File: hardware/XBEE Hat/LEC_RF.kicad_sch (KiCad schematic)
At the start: 6 parts, among them J1 Conn_Coaxial_Small, J2 Conn_01x04, U1 XBee_SMT, U2 TLV1117-33

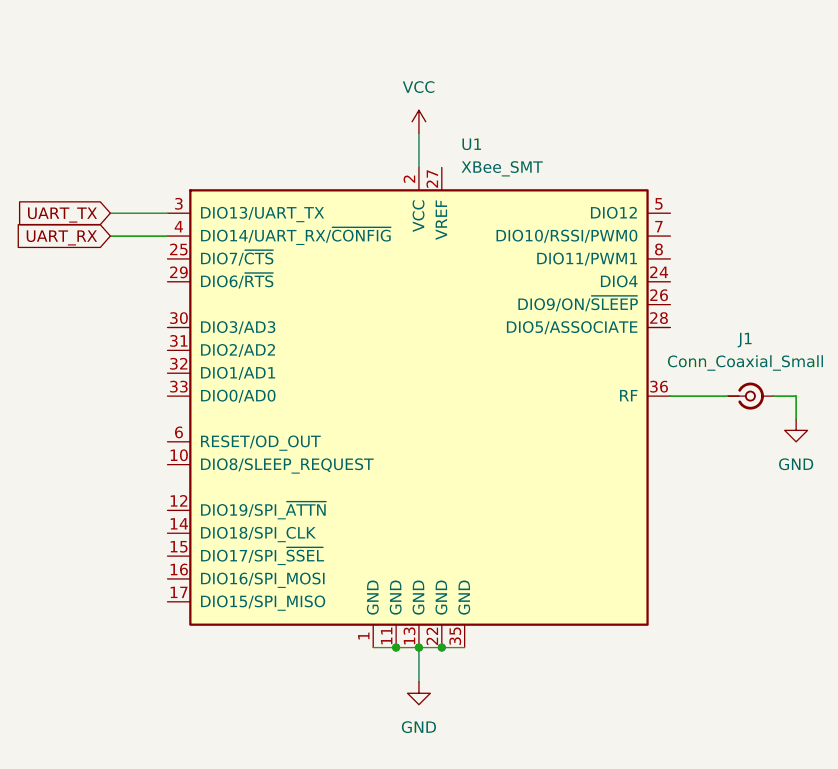
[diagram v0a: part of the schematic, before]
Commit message: Push of most recent schematic and PCB
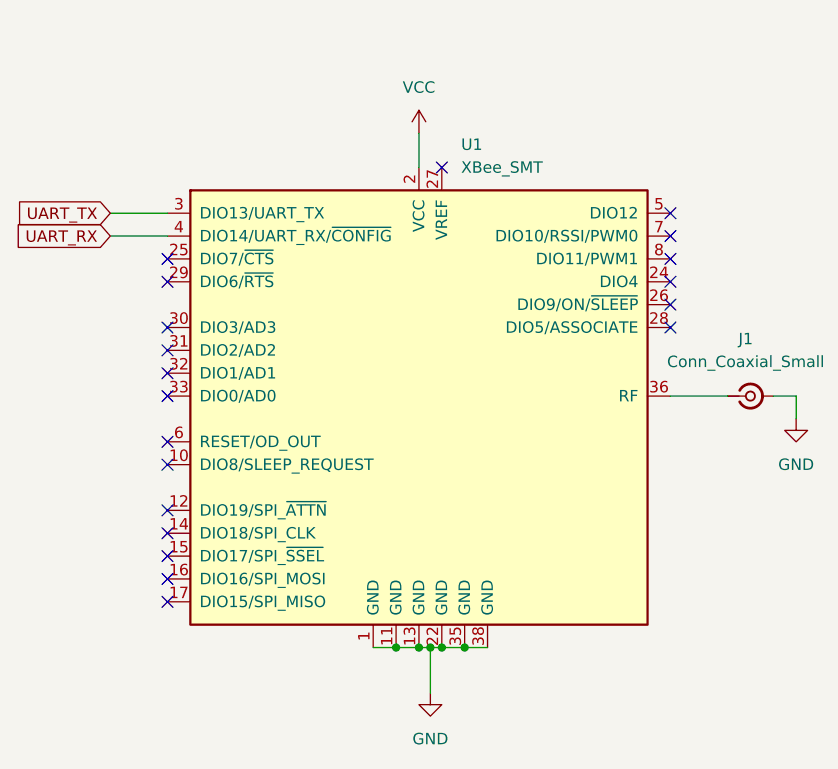
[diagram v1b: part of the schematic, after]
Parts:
- C1, C2: footprint Capacitor_SMD:C_0805_2012Metric -> Capacitor_SMD:C_0603_1608Metric
- U1: footprint RF_Module:Digi_XBee_SMT -> Custom:XBEE_GND_PAD
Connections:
- net GND: now also U1.38 (GND)
- no-connect marks 0 -> 20
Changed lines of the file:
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@@
 	(paper "A4")
+	(junction
+		(at 223.52 109.22)
+		(diameter 0)
+		(color 0 0 0 0)
+	)
+	(junction
+		(at 219.71 109.22)
+		(diameter 0)
+		(color 0 0 0 0)
+	)
 	(junction
 		(at 220.98 109.22)
@@
 		(color 0 0 0 0)
 	)
+	(no_connect
+		(at 190.5 99.06)
+	)
+	(no_connect
+		(at 190.5 93.98)
+	)
+	(no_connect
+		(at 190.5 88.9)
+	)
+	(no_connect
+		(at 190.5 96.52)
+	)
+	(no_connect
+		(at 220.98 55.88)
+	)
+	(no_connect
+		(at 190.5 68.58)
+	)
+	(no_connect
+		(at 246.38 60.96)
+	)
+	(no_connect
+		(at 246.38 63.5)
+	)
+	(no_connect
+		(at 246.38 71.12)
+	)
+	(no_connect
+		(at 190.5 101.6)
+	)
+	(no_connect
+		(at 246.38 68.58)
+	)
+	(no_connect
+		(at 190.5 66.04)
+	)
+	(no_connect
+		(at 190.5 81.28)
+	)
+	(no_connect
+		(at 190.5 73.66)
+	)
+	(no_connect
+		(at 246.38 73.66)
+	)
+	(no_connect
+		(at 246.38 66.04)
+	)
+	(no_connect
+		(at 190.5 76.2)
+	)
+	(no_connect
+		(at 190.5 86.36)
+	)
+	(no_connect
+		(at 190.5 78.74)
+	)
+	(no_connect
+		(at 190.5 104.14)
+	)
 	(wire
 		(pts
@@
 	(wire
 		(pts
-			(xy 218.44 109.22) (xy 218.44 113.03)
-		)
-		(stroke
-			(width 0)
-			(type default)
-		)
-	)
-	(wire
-		(pts
 			(xy 156.21 33.02) (xy 166.37 33.02)
 		)
@@
 	(wire
 		(pts
-			(xy 218.44 109.22) (xy 220.98 109.22)
+			(xy 218.44 109.22) (xy 219.71 109.22)
 		)
 		(stroke
@@
 	(wire
 		(pts
+			(xy 223.52 109.22) (xy 226.06 109.22)
+		)
+		(stroke
+			(width 0)
+			(type default)
+		)
+	)
+	(wire
+		(pts
 			(xy 144.78 33.02) (xy 156.21 33.02)
 		)
@@
 	(wire
 		(pts
+			(xy 219.71 109.22) (xy 220.98 109.22)
+		)
+		(stroke
+			(width 0)
+			(type default)
+		)
+	)
+	(wire
+		(pts
 			(xy 220.98 109.22) (xy 223.52 109.22)
 		)
@@
 		(pts
 			(xy 184.15 60.96) (xy 190.5 60.96)
+		)
+		(stroke
+			(width 0)
+			(type default)
+		)
+	)
+	(wire
+		(pts
+			(xy 219.71 109.22) (xy 219.71 114.3)
 		)
 		(stroke
@@
 	(symbol
 		(lib_id "power:GND")
-		(at 218.44 113.03 0)
+		(at 219.71 114.3 0)
 		(unit 1)
 		(exclude_from_sim no)
@@
 		(fields_autoplaced yes)
 		(property "Reference" "#PWR01"
-			(at 218.44 119.38 0)
+			(at 219.71 120.65 0)
 			(effects
 				(font
@@
 		)
 		(property "Value" "GND"
-			(at 218.44 118.11 0)
+			(at 219.71 119.38 0)
 			(effects
 				(font
@@
 		)
 		(property "Footprint" ""
-			(at 218.44 113.03 0)
+			(at 219.71 114.3 0)
 			(effects
 				(font
@@
 		)
 		(property "Datasheet" ""
-			(at 218.44 113.03 0)
+			(at 219.71 114.3 0)
 			(effects
 				(font
@@
 		)
 		(property "Description" "Power symbol creates a global label with name \"GND\" , ground"
-			(at 218.44 113.03 0)
+			(at 219.71 114.3 0)
 			(effects
 				(font
@@
 			)
 		)
-		(property "Footprint" "Capacitor_SMD:C_0805_2012Metric"
+		(property "Footprint" "Capacitor_SMD:C_0603_1608Metric"
 			(at 156.21 38.1 0)
 			(effects
@@
 			)
 		)
-		(property "Footprint" "RF_Module:Digi_XBee_SMT"
+		(property "Footprint" "Custom:XBEE_GND_PAD"
 			(at 239.776 108.204 0)
 			(effects
@@
 		)
 		(pin "36"
+		)
+		(pin "38"
 		)
 		(instances
@@
 			)
 		)
-		(property "Footprint" "Capacitor_SMD:C_0805_2012Metric"
+		(property "Footprint" "Capacitor_SMD:C_0603_1608Metric"
 			(at 144.78 38.1 0)
 			(effects
